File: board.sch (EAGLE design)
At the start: 86 parts, among them J1 AVR_SPI_PRG_6NS, U1 TPS2112A, U2 MAX1555, U3 USD-SOCKETNEW, U4 3.3V, U5 2.8V, U6 74HC595, Y1 8MHz, Y2 12.288MHz

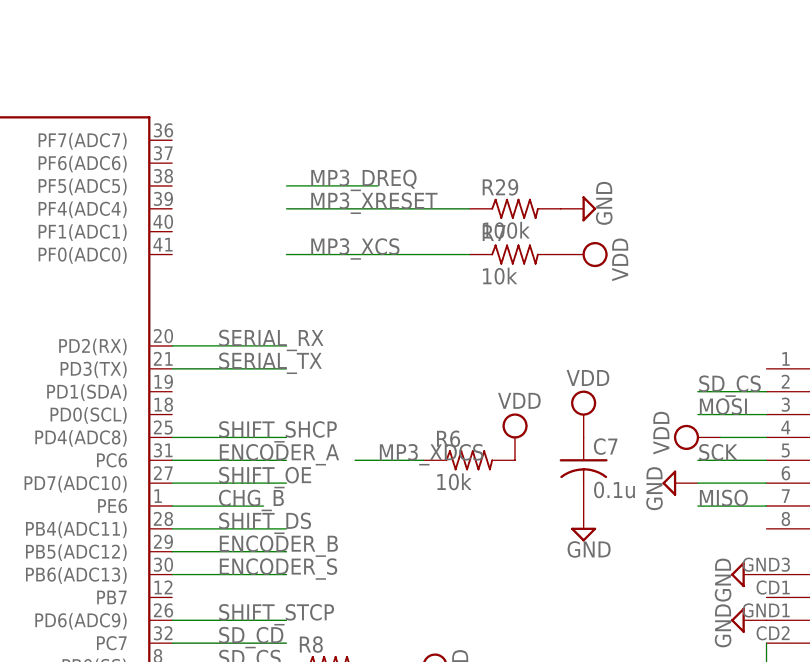
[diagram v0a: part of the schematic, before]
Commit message: Rough connections are made.
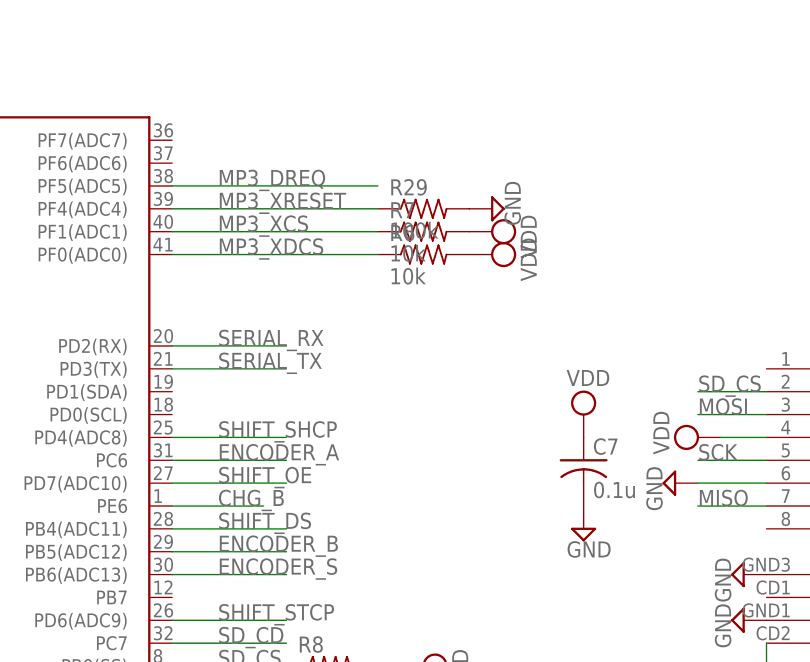
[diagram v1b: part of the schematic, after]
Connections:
- net MP3_DREQ: now also U$1.PF5(ADC5)
- net MP3_XCS: now also U$1.PF1(ADC1)
- net MP3_XDCS: now also U$1.PF0(ADC0)
- net MP3_XRESET: now also U$1.PF4(ADC4)
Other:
- moved on the sheet: R29, R6, R7
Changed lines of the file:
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@@
 <instance part="R13" gate="G$1" x="187.96" y="27.94" rot="R90"/>
 <instance part="SUPPLY10" gate="GND" x="180.34" y="20.32"/>
-<instance part="R7" gate="G$1" x="104.14" y="88.9"/>
+<instance part="R7" gate="G$1" x="93.98" y="91.44"/>
 <instance part="R8" gate="G$1" x="83.82" y="43.18"/>
-<instance part="R6" gate="G$1" x="99.06" y="66.04"/>
-<instance part="SUPPLY14" gate="G$1" x="104.14" y="68.58"/>
-<instance part="SUPPLY19" gate="G$1" x="111.76" y="88.9" rot="R270"/>
+<instance part="R6" gate="G$1" x="93.98" y="88.9"/>
+<instance part="SUPPLY14" gate="G$1" x="101.6" y="88.9" rot="R270"/>
+<instance part="SUPPLY19" gate="G$1" x="101.6" y="91.44" rot="R270"/>
 <instance part="SUPPLY52" gate="G$1" x="93.98" y="43.18" rot="R270"/>
-<instance part="R29" gate="G$1" x="104.14" y="93.98"/>
-<instance part="SUPPLY34" gate="GND" x="111.76" y="93.98" rot="R90"/>
+<instance part="R29" gate="G$1" x="93.98" y="93.98"/>
+<instance part="SUPPLY34" gate="GND" x="101.6" y="93.98" rot="R90"/>
 <instance part="U$1" gate="G$1" x="48.26" y="66.04"/>
 <instance part="SUPPLY53" gate="G$1" x="27.94" y="99.06" rot="R90"/>
@@
 <net name="MP3_XCS" class="0">
 <segment>
-<label x="81.28" y="88.9" size="1.778" layer="95"/>
+<label x="71.12" y="91.44" size="1.778" layer="95"/>
 <pinref part="R7" gate="G$1" pin="1"/>
-<wire x1="99.06" y1="88.9" x2="78.74" y2="88.9" width="0.1524" layer="91"/>
+<wire x1="88.9" y1="91.44" x2="66.04" y2="91.44" width="0.1524" layer="91"/>
+<pinref part="U$1" gate="G$1" pin="PF1(ADC1)"/>
 </segment>
 <segment>
@@
 </segment>
 <segment>
-<wire x1="86.36" y1="66.04" x2="93.98" y2="66.04" width="0.1524" layer="91"/>
-<label x="88.9" y="66.04" size="1.778" layer="95"/>
+<wire x1="66.04" y1="88.9" x2="88.9" y2="88.9" width="0.1524" layer="91"/>
+<label x="71.12" y="88.9" size="1.778" layer="95"/>
 <pinref part="R6" gate="G$1" pin="1"/>
+<pinref part="U$1" gate="G$1" pin="PF0(ADC0)"/>
 </segment>
 </net>
@@
 </segment>
 <segment>
-<wire x1="78.74" y1="96.52" x2="88.9" y2="96.52" width="0.1524" layer="91"/>
-<label x="81.28" y="96.52" size="1.778" layer="95"/>
+<label x="71.12" y="96.52" size="1.778" layer="95"/>
+<pinref part="U$1" gate="G$1" pin="PF5(ADC5)"/>
+<wire x1="88.9" y1="96.52" x2="66.04" y2="96.52" width="0.1524" layer="91"/>
 </segment>
 </net>
@@
 </segment>
 <segment>
-<label x="81.28" y="93.98" size="1.778" layer="95"/>
-<wire x1="78.74" y1="93.98" x2="99.06" y2="93.98" width="0.1524" layer="91"/>
+<label x="71.12" y="93.98" size="1.778" layer="95"/>
+<wire x1="66.04" y1="93.98" x2="88.9" y2="93.98" width="0.1524" layer="91"/>
 <pinref part="R29" gate="G$1" pin="1"/>
-</segment>
-</net>
+<pinref part="U$1" gate="G$1" pin="PF4(ADC4)"/>
+</segment>
+</net>
